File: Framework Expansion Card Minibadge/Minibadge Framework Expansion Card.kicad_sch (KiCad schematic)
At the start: 12 parts, among them P1 Connector_USB_C_Plug_USB2.0, U1 AP2112K-3.3

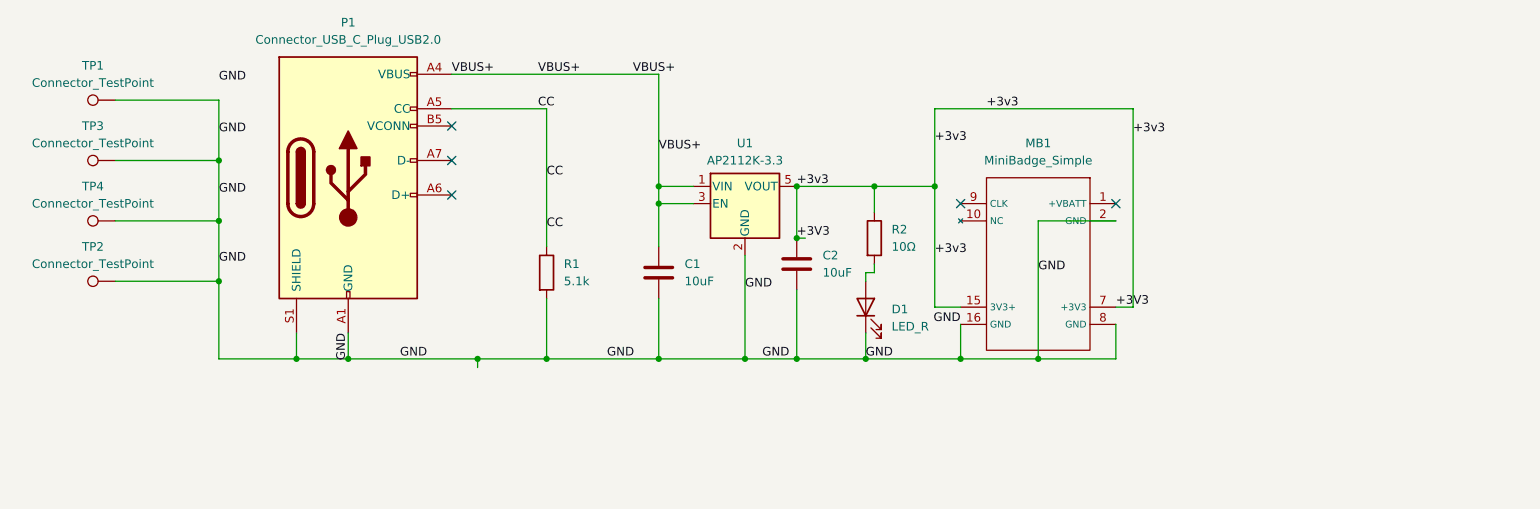
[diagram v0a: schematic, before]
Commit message: Add files via upload
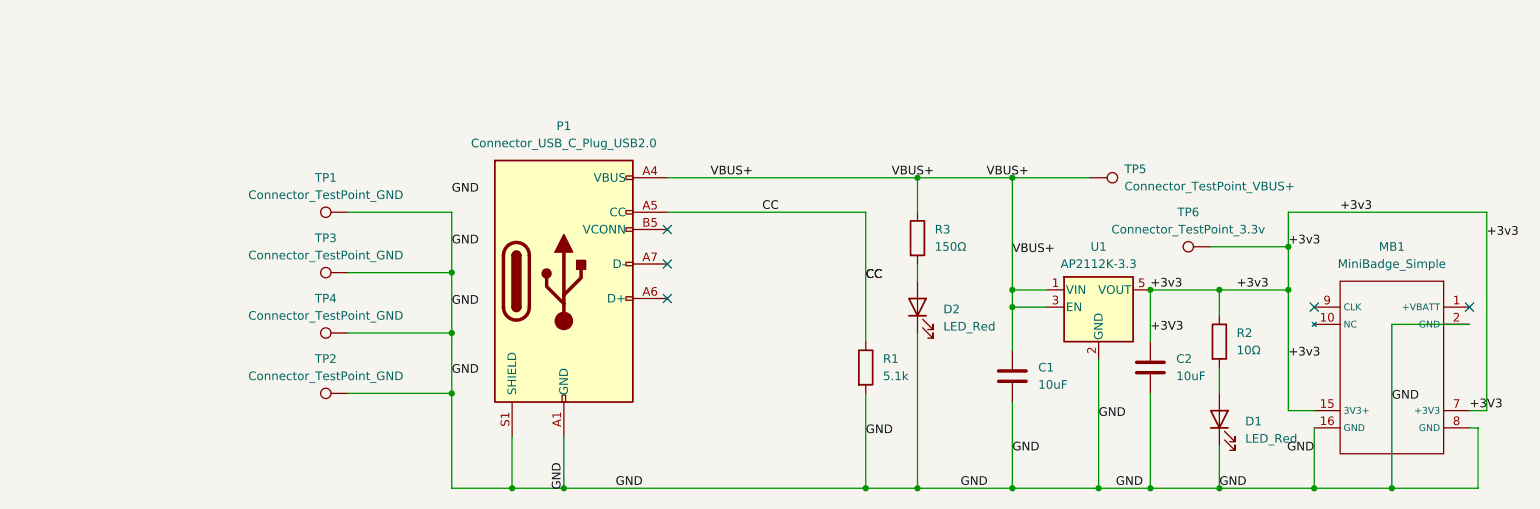
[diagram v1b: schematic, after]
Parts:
- added D2: LED_Red, LED_SMD:LED_1206_3216Metric_Pad1.42x1.75mm_HandSolder, symbol Device:LED
- added R3: 150Ω, Resistor_SMD:R_1206_3216Metric_Pad1.30x1.75mm_HandSolder, symbol Device:R
- added TP5: Connector_TestPoint_VBUS+, TestPoint:TestPoint_Pad_1.0x1.0mm, symbol Minibadge Framework Expansion Card-cache:Connector_TestPoint
- added TP6: Connector_TestPoint_3.3v, TestPoint:TestPoint_Pad_1.0x1.0mm, symbol Minibadge Framework Expansion Card-cache:Connector_TestPoint
- D1: value LED_R -> LED_Red
- TP1, TP2, TP3, TP4: value Connector_TestPoint -> Connector_TestPoint_GND
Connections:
- net +3V3: now also TP6.1
- net GND: now also D2.1 (K)
- net VBUS+: now also R3.1, TP5.1
- new net: D2.2 (A), R3.2
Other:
- moved on the sheet: C1, C2, D1, MB1, P1, R1, R2, TP1, TP2, TP3, TP4, U1
